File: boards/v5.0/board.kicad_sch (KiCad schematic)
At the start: 11 parts, among them J1 Screw_Terminal_01x02, J2 Screw_Terminal_01x04, J3 Screw_Terminal_01x02, J4 Screw_Terminal_01x02, J5 Screw_Terminal_01x02, J6 Screw_Terminal_01x02, P4 Pin Header, P5 Pin Header, P6 Conn_01x07, P7 Pin Header, P8 Pin Header

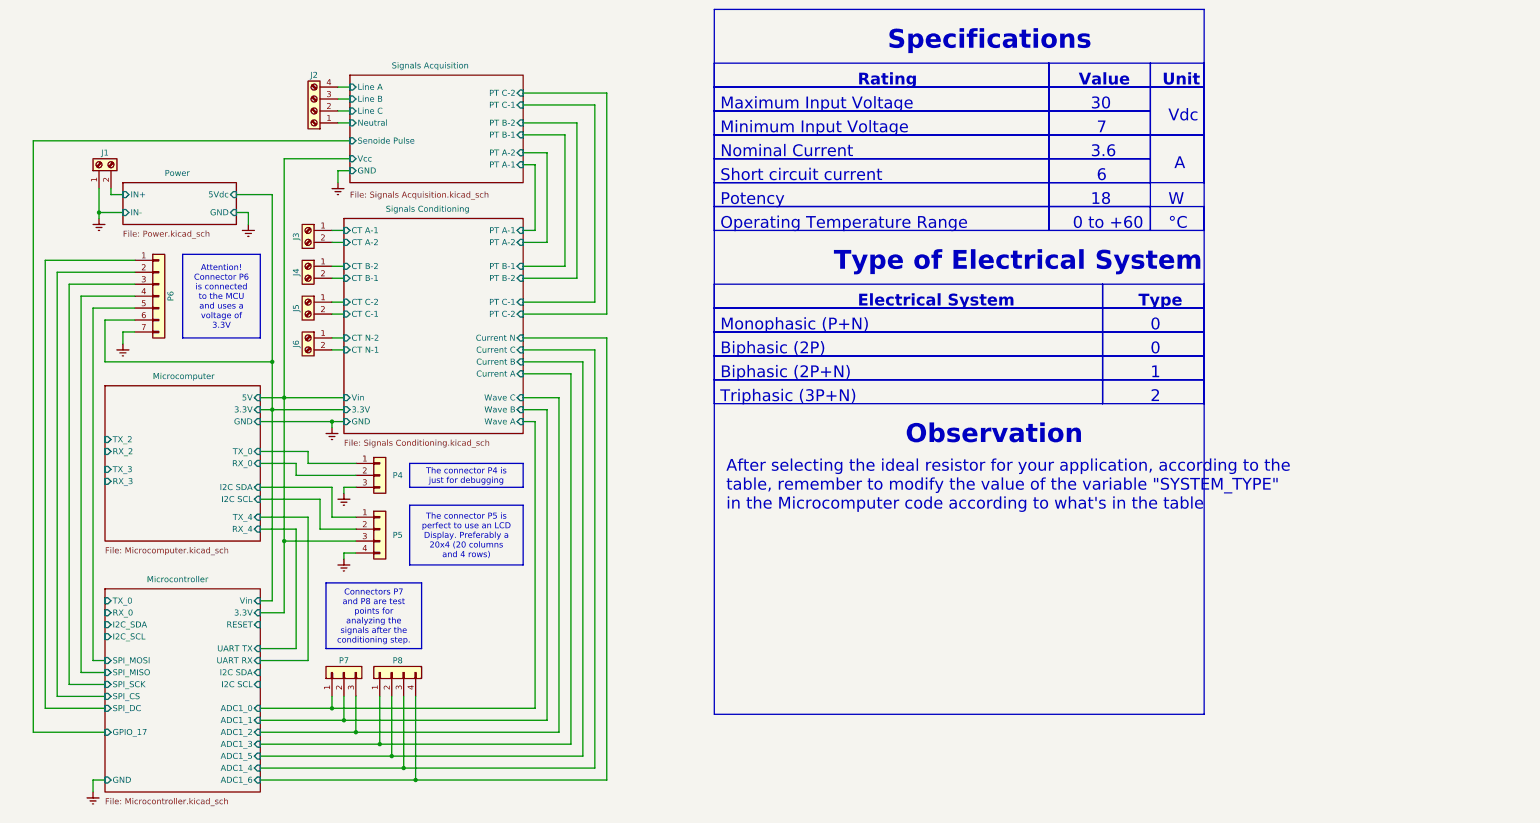
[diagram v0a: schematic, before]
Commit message: Update in the V5 board
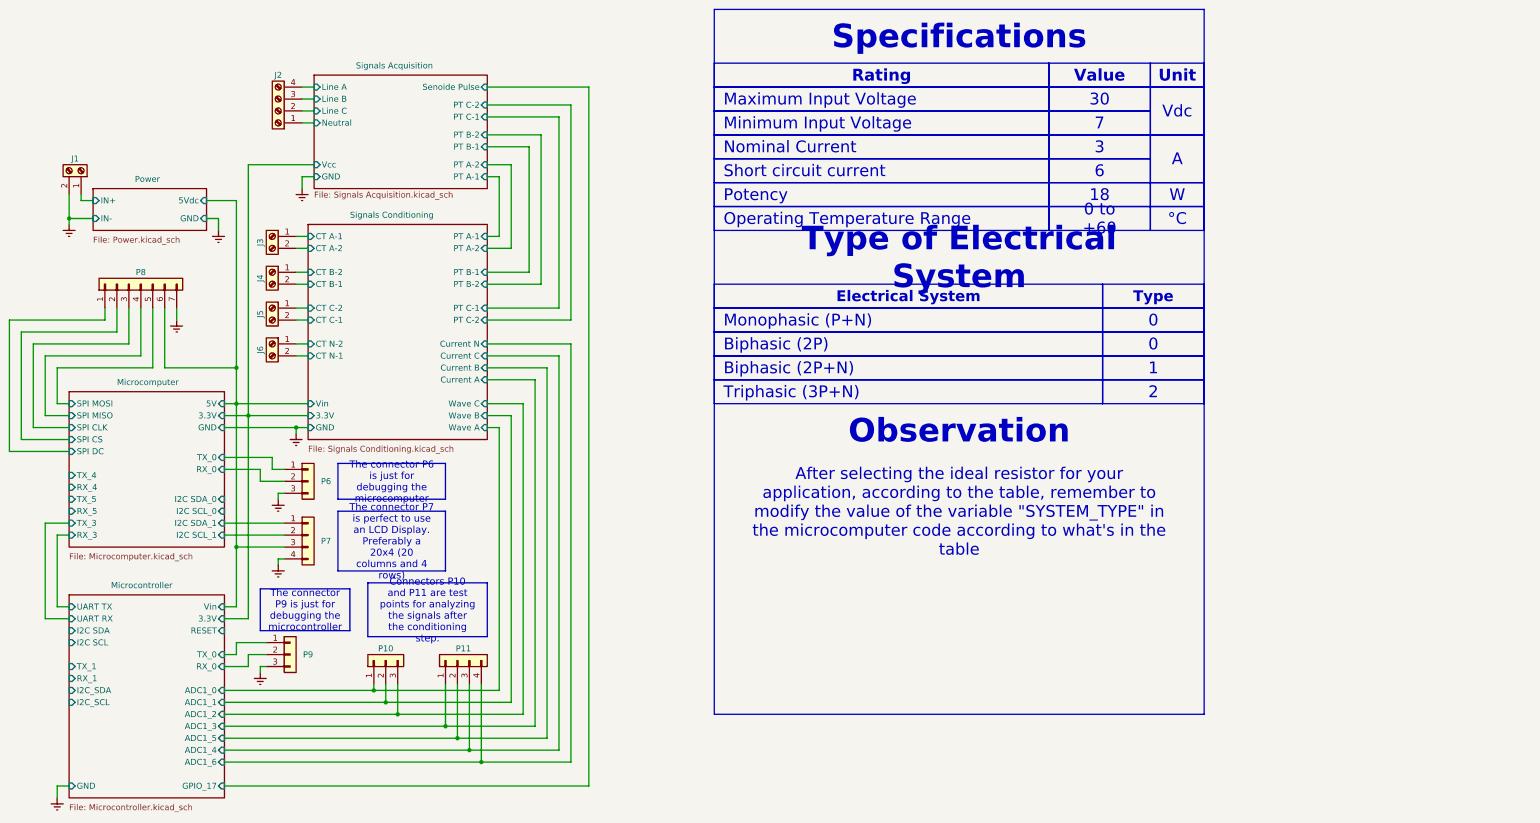
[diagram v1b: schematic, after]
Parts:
- added P9: Pin Header, Connector_PinHeader_2.54mm:PinHeader_1x03_P2.54mm_Vertical, symbol Connector_Generic:Conn_01x03
- renumbered P7 to P10, P8 to P11, P4 to P6, P5 to P7, P6 to P8
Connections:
- net Earth: now also J1.2 (Pin_2), P9.3 (Pin_3); no longer J1.1 (Pin_1)
- net Microcomputer/3.3V: no longer P8.6 (Pin_6)
- net Microcomputer/5V: now also P8.6 (Pin_6)
- net Microcontroller/RX_0: now also P9.2 (Pin_2)
- net Microcontroller/TX_0: now also P9.1 (Pin_1)
- net Power/IN+: now also J1.1 (Pin_1); no longer J1.2 (Pin_2)
- net Microcomputer/I2C SCL renamed Microcomputer/I2C SCL_1
- net Microcomputer/I2C SDA renamed Microcomputer/I2C SDA_1
- net Microcontroller/SPI_CS renamed Microcomputer/SPI CS
- net Microcontroller/SPI_DC renamed Microcomputer/SPI DC
- net Microcontroller/SPI_MISO renamed Microcomputer/SPI MISO
- net Microcontroller/SPI_MOSI renamed Microcomputer/SPI MOSI
- net Microcontroller/SPI_SCK renamed Microcomputer/SPI CLK
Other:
- sheet Microcomputer ports: added I2C SCL_0, I2C SCL_1, I2C SDA_0, I2C SDA_1, RX_5, SPI CLK, SPI CS, SPI DC, SPI MISO, SPI MOSI, TX_5; removed I2C SCL, I2C SDA, RX_2, TX_2
- sheet Microcontroller ports: added RX_1, TX_1; removed SPI_CS, SPI_DC, SPI_MISO, SPI_MOSI, SPI_SCK
- note removed: "0"
- note removed: "0 to +60"
- note removed: "1"
- note removed: "18"
- note removed: "2"
- note removed: "3.6"
- note removed: "30"
- note removed: "6"
- note removed: "7"
- note removed: "A"
- note removed: "After selecting the ideal resistor for your application, according to the table, remember to modify the value of the variable "SYSTEM_TYPE" in the Microcomputer code according to what's in the table"
- note removed: "Biphasic (2P)"
- note removed: "Biphasic (2P+N)"
- note removed: "Electrical System"
- note removed: "Maximum Input Voltage"
- note removed: "Minimum Input Voltage"
- note removed: "Monophasic (P+N)"
- note removed: "Nominal Current"
- note removed: "Observation"
- note removed: "Operating Temperature Range"
- note removed: "Potency"
- note removed: "Rating"
- note removed: "Short circuit current"
- note removed: "Specifications"
- note removed: "Triphasic (3P+N)"
- note removed: "Type"
- note removed: "Type of Electrical System"
- note removed: "Unit"
- note removed: "Value"
- note removed: "Vdc"
- note removed: "W"
- note removed: "°C"
- moved on the sheet: J1, J2, J3, J4, J5, J6, P10, P11, P6, P7, P8
